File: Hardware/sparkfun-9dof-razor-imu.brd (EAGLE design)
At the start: 40.6 x 27.9 mm, 40 parts, among them J1 AVR_SPI_PRG_6PTH, Q1 8MHz, U1 ITG-32001:1, U2 ADXL3451:1, U5 3.3V, U6 ATMEGA328

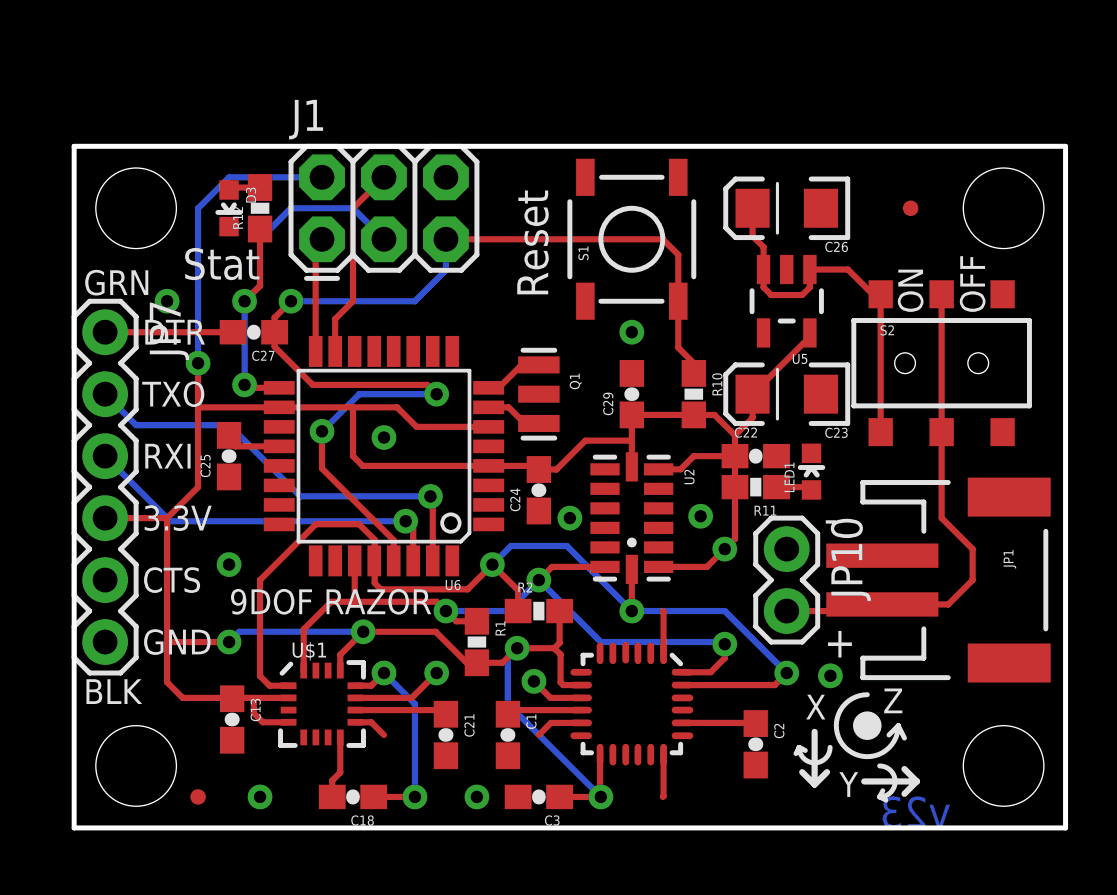
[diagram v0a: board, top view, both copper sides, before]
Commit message: Initial commit of v24.
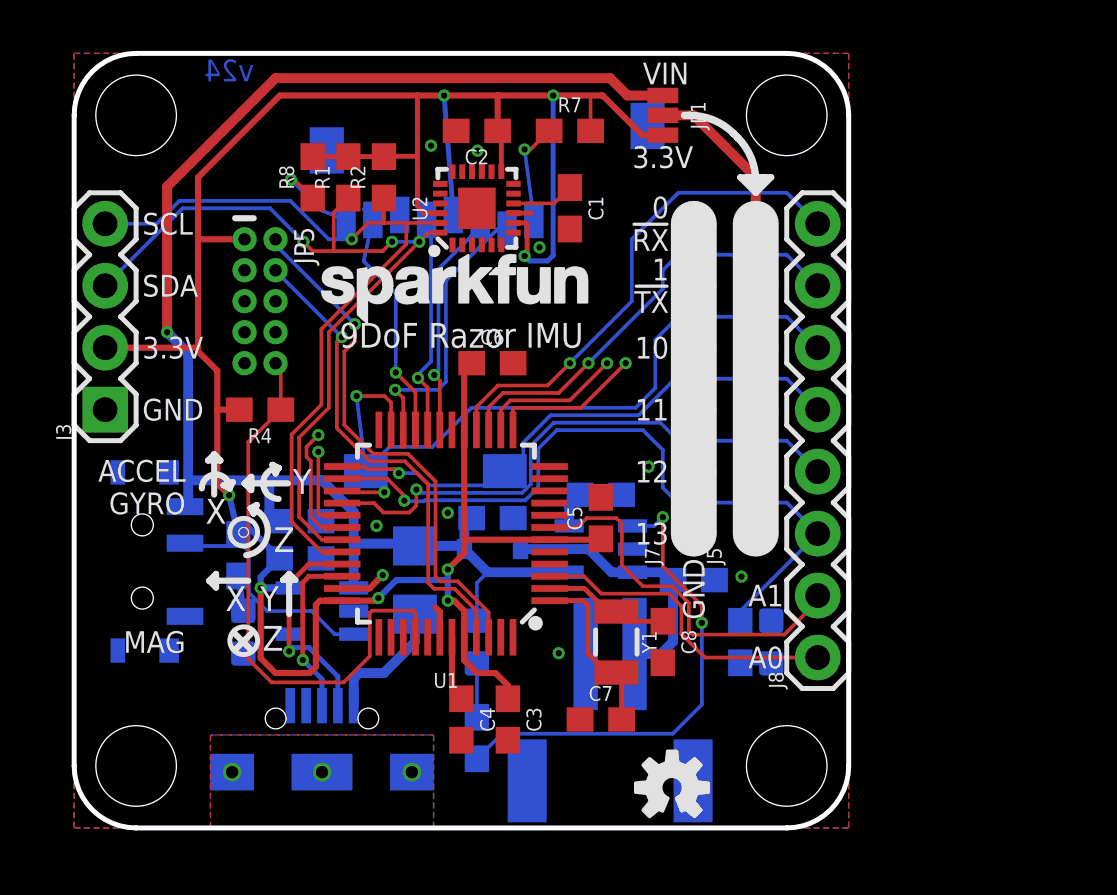
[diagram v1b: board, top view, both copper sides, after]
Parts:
- removed C13, C22, C24, C25, C27, C29: 0.1uF, SparkFun:0603-CAP
- removed C18: 0.22uF, SparkFun:0603-CAP
- removed C21: 4.7uF, SparkFun:0603-CAP
- removed C23, C26: 10uF, SparkFun:EIA3216
- removed JP10: JST_Horizontal, SparkFun:1X02
- removed JP11, JP12: FIDUCIAL1X2.5, abes:FIDUCIAL-1X2.5
- removed JP2, JP4, JP6: STAND-OFF, SparkFun:STAND-OFF
- removed JP3: LOGO-SFENEW, SparkFun:SFE-NEW-WEBLOGO
- removed JP7: FTDI Basic, SparkFun:1X06
- removed LED1: Red, SparkFun:LED-0603
- removed Q1: 8MHz, SparkFun:RESONATOR-SMD
- removed R11: 10K, SparkFun:0603-RES
- removed R12: 330, SparkFun:0603-RES
- removed S2: Power, SparkFun:AYZ0202
- removed U$1: HMC5883LSMD, SparkFun:16LPCC
- removed U$4: OSHW-LOGOL, SparkFun:OSHW-LOGO-L
- removed U5: 3.3V, SparkFun:SOT23-5
- removed U6: ATMEGA328, SparkFun:TQFP32-08
- added C10: 2.2uF, SparkFun-Capacitors:0603
- added C11, C12: 4.7uF, SparkFun-Capacitors:0603
- added C4, C5, C6: 0.1uF, SparkFun-Capacitors:0603
- added C7, C8: 15pF, SparkFun-Capacitors:0603
- added C9: 1.0uF, SparkFun-Capacitors:0603
- added D1: 1A/23V/620mV, SparkFun-DiscreteSemi:SOD-323
- added D2: RED, SparkFun-LED:LED-0603
- added D4: Yellow, SparkFun-LED:LED-0603
- added F1: 6V/0.5A, SparkFun-Fuses:1206
- added FRAME1: FRAME-LEDGER, SparkFun-Aesthetics:CREATIVE_COMMONS
- added H1, H2, H3, H4: STAND-OFF, SparkFun-Electromechanical:STAND-OFF
- added J2: (no value), SparkFun-Connectors:JST-2-SMD
- added J3: (no value), SparkFun-Connectors:1X04
- added J4: (no value), SparkFun-Connectors:USB-B-MICRO-SMD_V03
- added J5, J7: (no value), SparkFun-Connectors:1X06_NO_SILK
- added J8: (no value), SparkFun-Connectors:1X08
- added LOGO1: SFE_LOGO_FLAME.1_INCH, SparkFun-Aesthetics:SFE_LOGO_FLAME_.1
- added LOGO2: OSHW-LOGOS, SparkFun-Aesthetics:OSHW-LOGO-S
- added LOGO3: SFE_LOGO_NAME.1_INCH, SparkFun-Aesthetics:SFE_LOGO_NAME_.1
- added R3, R5: 1k, SparkFun-Resistors:0603
- added R4: 10k, SparkFun-Resistors:0603
- added R7, R8: 100k, SparkFun-Resistors:0603
- added R9: 2.2k, SparkFun-Resistors:0603
- added U3: 3.3V, SparkFun-IC-Power:SOT23-5
- added U4: MCP73831, SparkFun-IC-Power:SOT23-5
- added Y1: 32.768kHz, SparkFun-Clocks:CRYSTAL-SMD-3.2X1.5MM
- C1: device SparkFun:0603-CAP -> SparkFun-Capacitors:0603
- C2: value 2.2nF -> 0.1uF; device SparkFun:0603-CAP -> SparkFun-Capacitors:0603
- C3: value 10nF -> 0.1uF; device SparkFun:0603-CAP -> SparkFun-Capacitors:0603
- D3: value Green -> BLUE; device SparkFun:LED-0603 -> SparkFun-LED:LED-0603
- J1: value AVR_SPI_PRG_6PTH -> USD_CONNECTOR; device SparkFun:2X3 -> SparkFun-Connectors:MICRO-SD-SOCKET-PP
- JP1: value JST_Horizontal -> PWR-SELECT; device SparkFun:JST-2-SMD -> SparkFun-Jumpers:SMT-JUMPER_3_1-NC_PASTE_NO-SILK
- JP5: value STAND-OFF -> CORTEX_DEBUGPTH; device SparkFun:STAND-OFF -> samd21-temp:2X5-PTH-1.27MM
- R1: device SparkFun:0603-RES -> SparkFun-Resistors:0603
- R10: value 10K -> 1k; device SparkFun:0603-RES -> SparkFun-Resistors:0603
- R2: value 4.7K -> 4.7k; device SparkFun:0603-RES -> SparkFun-Resistors:0603
- S1: value Reset -> (none); device SparkFun:TACTILE_SWITCH_SMD -> SparkFun-Electromechanical:SWITCH-SPST-SMD-A
- U1: value ITG-32001:1 -> ATSAMD21G-A; device Testing:QFN-24_ITG3200_1:1 -> SparkFun-IC-Microcontroller:TQFP-48
- U2: value ADXL3451:1 -> MPU-9250"; device Testing:LGA14 -> 9dof-devboard-temp:QFN24-3X3
- moved JP5 30.7 mm to (7.62, 21.6), turned to 270 degrees
- moved D3 28.5 mm to (28.6, 7.62), flipped to the bottom, turned to 90 degrees
- moved C2 27.6 mm to (16.5, 28.6), turned to 180 degrees
- moved S1 24.0 mm to (2.79, 10.9), flipped to the bottom, turned to 270 degrees
- moved JP1 22.9 mm to (24.1, 29.2)
- moved C1 21.7 mm to (20.3, 25.4)
- moved R1 19.8 mm to (11.2, 26.7), turned to 90 degrees
- moved R2 18.9 mm to (12.7, 26.7), turned to 90 degrees
- moved R10 16.7 mm to (16.5, 3.68), flipped to the bottom, turned to 90 degrees
- moved U2 14.2 mm to (16.5, 25.4), turned to 90 degrees
- moved U1 10.3 mm to (15.2, 12.1), turned to 180 degrees
- moved J1 9.91 mm to (9.91, 14.2), flipped to the bottom
- moved C3 3.42 mm to (17.8, 4.45), turned to 270 degrees
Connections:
- removed net DTR: C27.2, JP7.1
- removed net MISO: J1.1, U6.16
- removed net MOSI: J1.4, U6.15
- removed net N$12: D3.A, R12.2
- removed net N$13: Q1.1, U6.8
- removed net N$14: Q1.3, U6.7
- removed net N$15: JP1.2, JP10.2, S2.2, S2.5
- removed net N$38: LED1.A, R11.1
- removed net RAW: C26.A, S2.1, S2.4, U5.1, U5.3
- removed net RESET: C27.1, J1.5, R10.1, S1.3, U6.29
- removed net RXI: JP7.3, U6.30
- removed net SCK: J1.3, R12.1, U6.17
- removed net TXO: JP7.2, U6.31
- new net !RESET: JP5.10, R4.1, U1.40
- new net A0: J8.1, U1.3
- new net A1: J8.2, U1.7
- new net A2: U1.8
- new net A3: U1.9
- new net A4: U1.10
- new net A5: U1.47
- new net CHG_LED: R10.1, U4.1
- new net D0/RXI: J8.8, U1.16
- new net D1/TXO: J8.7, U1.15
- new net D10: J8.6, U1.27
- new net D11: J8.5, U1.25
- new net D12: J8.4, U1.28
- new net D13: J8.3, R3.2, U1.26
- new net D2/SD_CD: J1.CD1, U1.23
- new net D3: U1.14
- new net D4: U1.13
- new net D5: U1.24
- new net D6: U1.29
- new net D7: U1.30
- new net D8: U1.11
- new net D9: U1.12
- new net FSYNC: U2.11
- new net INT: U2.12
- new net N$10: C11.1, D1.A, J2.2, U4.3
- new net N$11: D4.C, R10.2
- new net N$5: D2.A, R5.1
- new net N$7: R9.2, U4.5
- new net N$8: J1.RSV1, R7.1
- new net N$9: J1.RSV2, R8.1
- new net REGOUT: C1.1, U2.10
- new net RX_EDBG: U1.38
- new net RX_LED: U1.48
- new net SD_!CS!: J1.CS, U1.22
- new net SD_MISO: J1.DO, U1.21
- new net SD_MOSI: J1.DI, U1.19
- new net SD_SCK: J1.SCLK, U1.20
- new net SHIELD: J4.SHIELD1, J4.SHIELD2, J4.SHIELD3
- new net SWCLK: JP5.4, U1.45
- new net SWDIO: JP5.2, U1.46
- new net TX_EDBG: U1.37
- new net TX_LED: U1.39
- new net USB_D+: J4.D+, U1.34
- new net USB_D-: J4.D-, U1.33
- new net USB_HOST_EN: U1.41
- new net VDDCORE: C4.1, U1.43
- new net VIN: C12.1, C9.1, D1.C, D4.A, F1.2, JP1.1, S1.1, U3.1, U4.4
- new net VREG_EN: S1.2, U3.3
- net 3.3V: now also C10.1, C2.1, C5.1, C6.1, J1.VCC, J3.2, JP1.3, JP5.1, R4.2, R5.2, R7.2, R8.2, U1.17, U1.36, U1.44, U1.6, U2.13, U2.22, U2.8, U3.5; no longer C13.1, C22.1, C23.A, C24.2, C29.1, J1.2, JP7.4, R10.2, R11.2, U$1.13, U$1.2, U$1.4, U1.13, U1.8, U2.1, U2.6, U2.7, U5.5, U6.18, U6.4, U6.6
- net AREF: now also U1.4; no longer C25.2, U6.20
- net GND: now also C10.2, C11.2, C12.2, C4.2, C5.2, C6.2, C7.1, C8.2, C9.2, D2.C, J1.GND, J1.GND1, J1.GND3, J2.1, J3.1, J4.GND, J7.1, J7.2, J7.3, J7.4, J7.5, J7.6, JP5.3, JP5.5, R9.1, S1.3, U1.35, U1.42, U1.5, U2.18, U2.9, U3.2, U4.2; no longer C13.2, C21.2, C22.2, C23.C, C24.1, C25.1, C26.C, C29.2, J1.6, JP1.1, JP10.1, JP7.5, JP7.6, LED1.C, Q1.2, S1.1, U$1.11, U$1.9, U1.1, U1.11, U1.9, U2.12, U2.2, U2.4, U2.5, U5.2, U6.21, U6.3, U6.5
- net N$1: now also F1.1, J4.VBUS; no longer C18.2, U$1.8
- net N$2: now also C7.2, U1.1, Y1.P$2; no longer C18.1, U$1.12
- net N$3: now also D3.A, R3.1; no longer C1.1, U1.10
- net N$4: now also C8.1, U1.2, Y1.P$1; no longer C2.1, U1.20
- net N$6: now also J5.1, J5.2, J5.3, J5.4, J5.5, J5.6, JP1.2; no longer C21.1, U$1.10
- net SCL: now also J3.4, U1.32, U2.23; no longer U$1.1, U1.23, U2.14, U6.28
- net SDA: now also J3.3, U1.31, U2.24; no longer U$1.16, U1.24, U2.13, U6.27
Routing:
- net VIN: track 0.00 -> 61.8 mm, vias 0 -> 1
- net RESET: track 44.5 -> 0.00 mm, vias 3 -> 0
- net D13: track 0.00 -> 29.7 mm, vias 0 -> 1
- net D10: track 0.00 -> 25.1 mm, vias 0 -> 1
- net D12: track 0.00 -> 23.4 mm, vias 0 -> 1
- net !RESET: track 0.00 -> 23.3 mm
- net D11: track 0.00 -> 23.1 mm, vias 0 -> 1
- net SWDIO: track 0.00 -> 21.5 mm, vias 0 -> 1
- net D0/RXI: track 0.00 -> 20.6 mm, vias 0 -> 1
- net N$15: track 20.4 -> 0.00 mm
- net SWCLK: track 0.00 -> 20.0 mm, vias 0 -> 1
- net CHG_LED: track 0.00 -> 19.9 mm, vias 0 -> 2
- net D1/TXO: track 0.00 -> 18.0 mm, vias 0 -> 1
- net TXO: track 17.8 -> 0.00 mm, vias 1 -> 0
- net SCK: track 17.1 -> 0.00 mm, vias 2 -> 0
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- added copper zone on layer 1, net SHIELD
- added copper zone on layer 16, net SHIELD
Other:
- board size 40.6 x 27.9 mm -> 31.8 x 31.8 mm
- board text added: "0 !RX"
- board text added: "1 !TX"
- board text added: "10"
- board text added: "11"
- board text added: "12"
- board text added: "13"
- board text added: "9DoF Razor IMU"
- board text added: "A0"
- board text added: "A1"
- board text added: "ACCEL GYRO"
- board text added: "CHG"
- board text added: "MAG"
- board text added: "PWR"
- board text added: "SCL"
- board text added: "SDA"
- board text added: "VBUS"
- board text added: "VIN"
- board text added: "v24"
- board text removed: "+"
- board text removed: "-"
- board text removed: "9DOF RAZOR"
- board text removed: "BLK"
- board text removed: "CTS"
- board text removed: "DTR"
- board text removed: "GRN"
- board text removed: "RXI"
- board text removed: "Reset"
- board text removed: "Stat"
- board text removed: "TXO"
- board text removed: "v23"
